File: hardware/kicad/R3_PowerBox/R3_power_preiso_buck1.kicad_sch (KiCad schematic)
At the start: 19 parts, among them U2 TPS54302DDCR

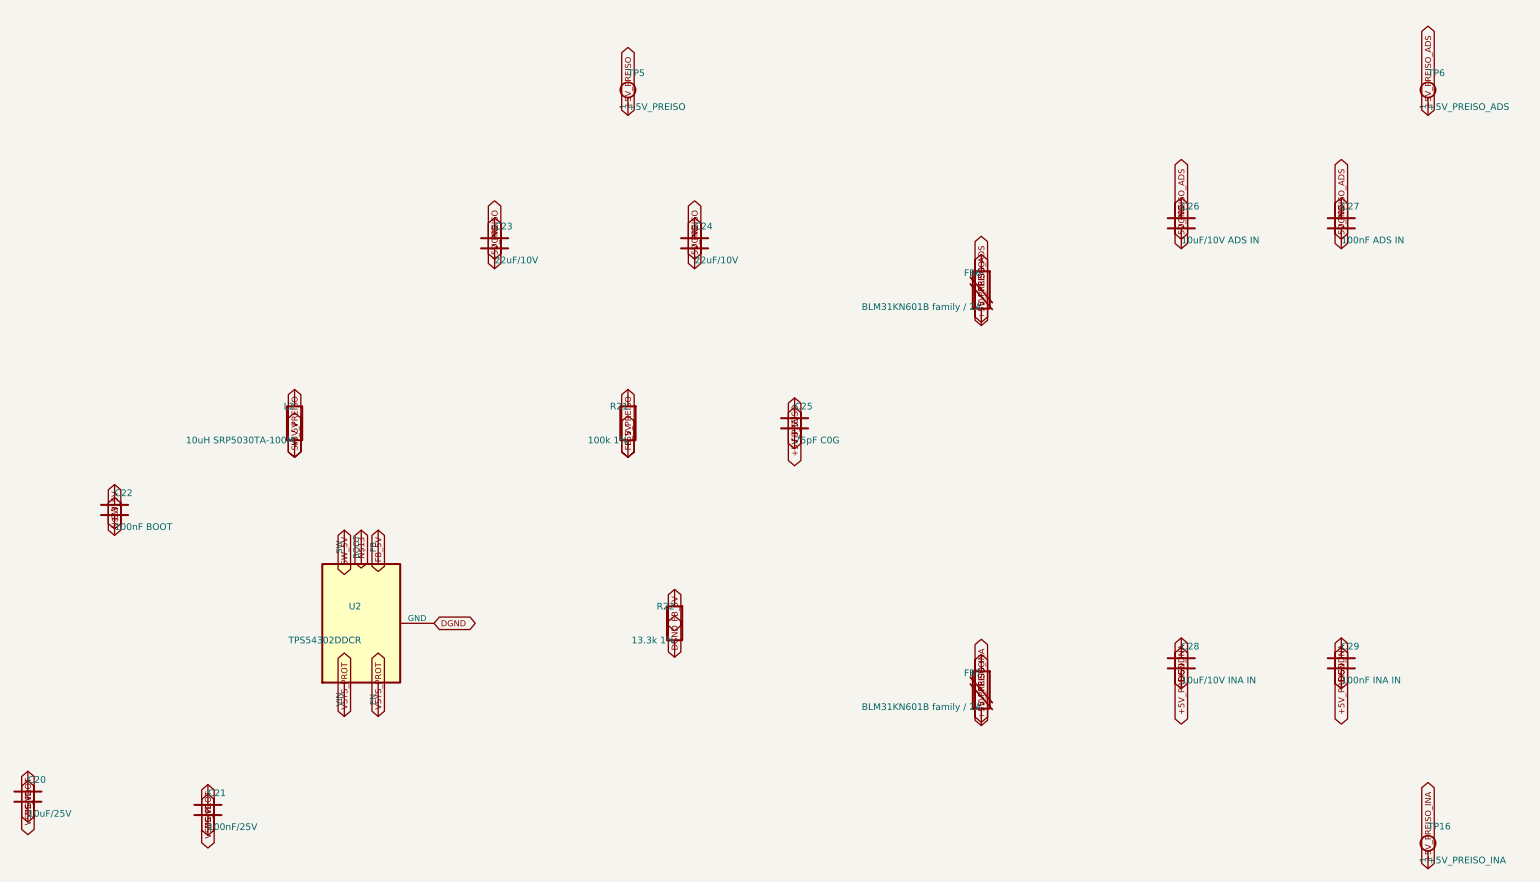
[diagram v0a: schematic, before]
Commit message: Finalize R3 PowerBox pre-placement corrections
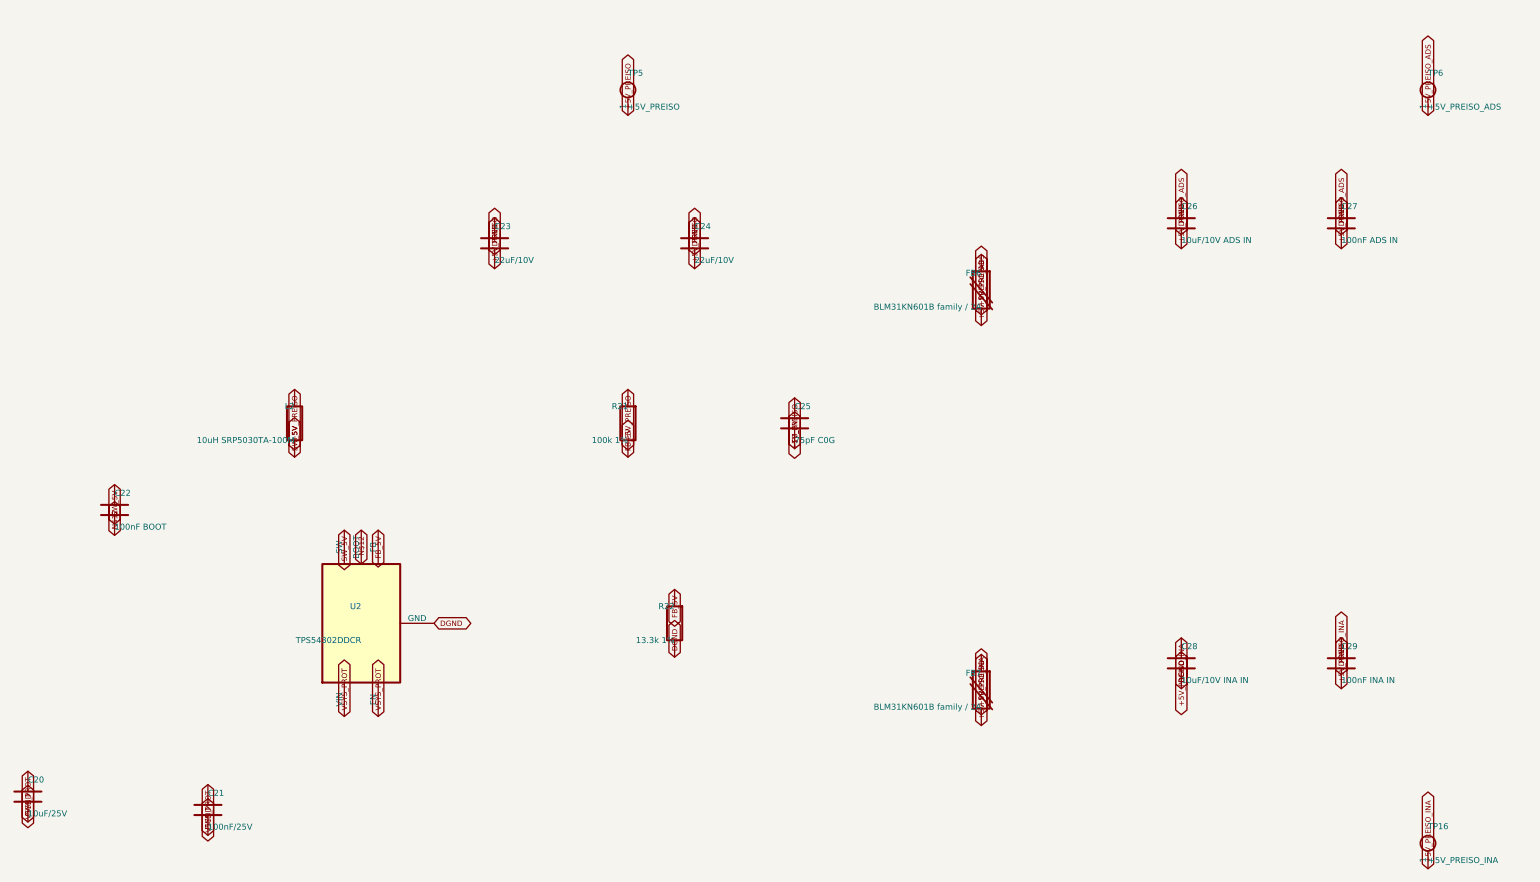
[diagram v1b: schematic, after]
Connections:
- net N$13 renamed N$12
